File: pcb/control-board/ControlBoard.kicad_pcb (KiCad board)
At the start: 2 copper layers, 71 parts, among them J1 BOOT0, J10 Motor8, J12 Motor9, J13 Motor10, J14 JTAG-SWD, J15 HEADER_L, J16 HEADER_D, J17 HEADER_U, J18 HEADER_R, J2 Motor1, J20 PWR, J3 Motor2, J4 Motor3, J5 Motor4, J6 Motor5, J7 Motor6, J8 Motor7, J9 USB_B_Micro, SW1 RST_BTN, U1 STM32F427VGTx, U2 USBLC6-2SC6, U3 MCP1700-3302E_SOT89, U4 FT230XS, Y1 8MHz, Y2 32.768kHz

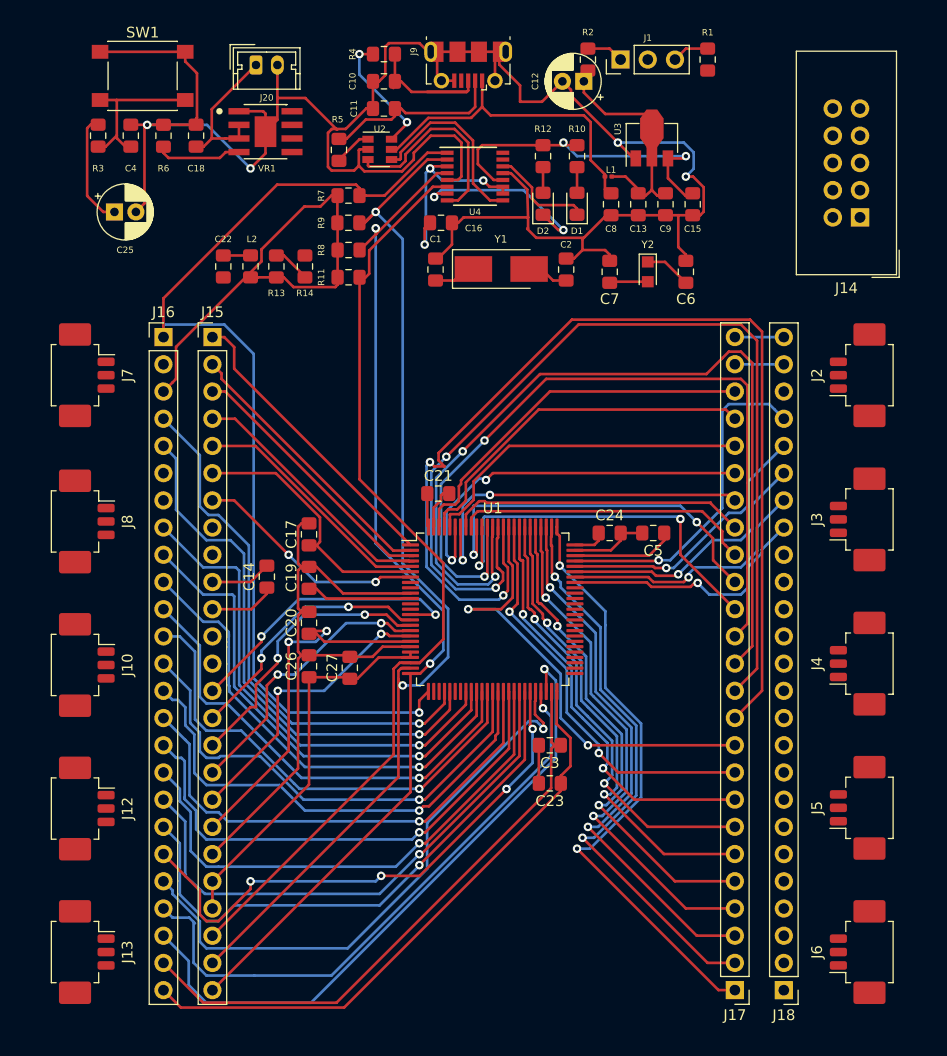
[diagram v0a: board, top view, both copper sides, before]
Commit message: Finish control board pcb
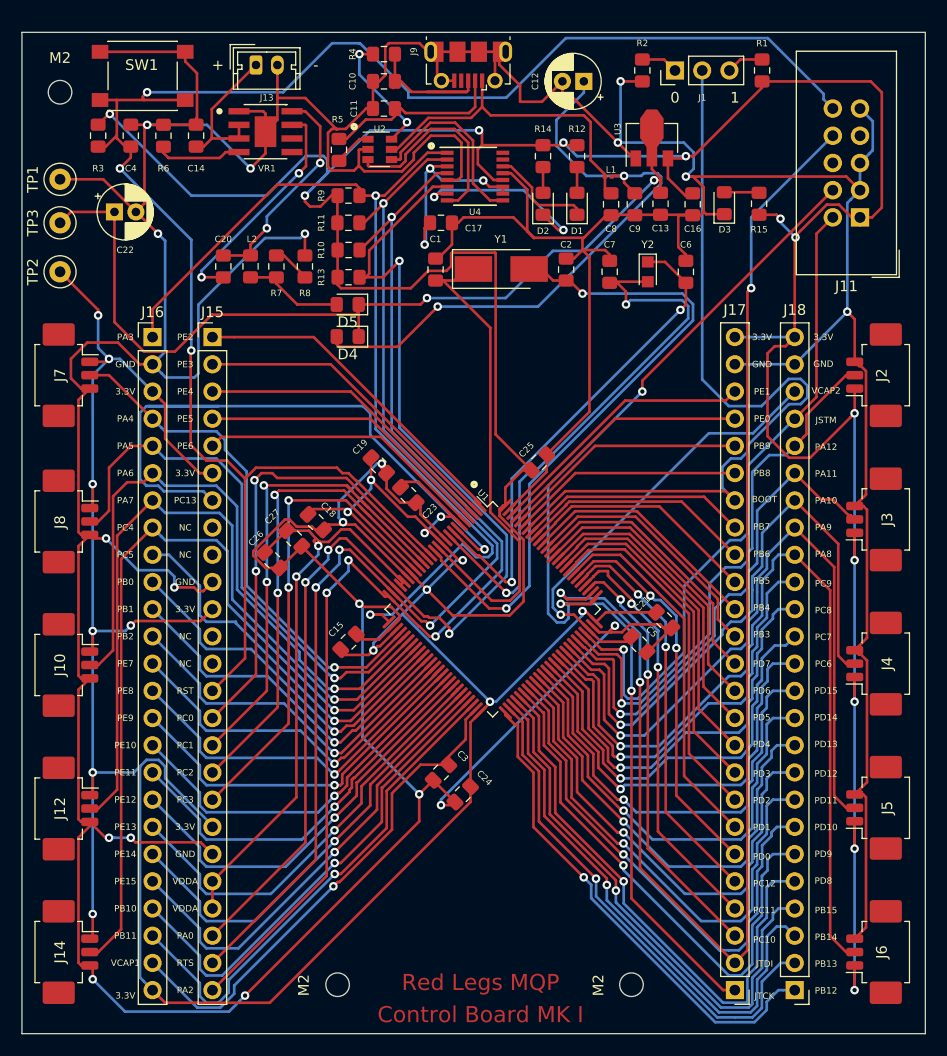
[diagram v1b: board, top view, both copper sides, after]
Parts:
- removed the C17 at (166.0, 97.7)
- removed the C23 at (188.5, 120.9)
- added C18: 100nF, Capacitor_SMD:C_0805_2012Metric_Pad1.15x1.40mm_HandSolder, F.Cu at (166.6, 96.5)
- added C24: 100nF, Capacitor_SMD:C_0805_2012Metric_Pad1.15x1.40mm_HandSolder, F.Cu at (180.3, 121.9)
- added D3: LED, LED_SMD:LED_0805_2012Metric_Pad1.15x1.40mm_HandSolder, F.Cu at (204.8, 66.8)
- added D4: SD0805, Diode_SMD:D_0805_2012Metric_Pad1.15x1.40mm_HandSolder, F.Cu at (169.6, 79.2)
- added D5: SD0805, Diode_SMD:D_0805_2012Metric_Pad1.15x1.40mm_HandSolder, F.Cu at (169.6, 76.2)
- added M2: MountingHole_2.2mm_M2, MountingHole:MountingHole_2.2mm_M2, F.Cu at (196.1, 139.7)
- added M2: MountingHole_2.2mm_M2, MountingHole:MountingHole_2.2mm_M2, F.Cu at (168.7, 139.7)
- added M2: MountingHole_2.2mm_M2, MountingHole:MountingHole_2.2mm_M2, F.Cu at (142.7, 56.4)
- added R15: 220, Resistor_SMD:R_0805_2012Metric_Pad1.15x1.40mm_HandSolder, F.Cu at (208.0, 66.8)
- added TP1: TestPoint, TestPoint:TestPoint_Loop_D2.50mm_Drill1.0mm, F.Cu at (142.7, 64.5)
- added TP2: TestPoint, TestPoint:TestPoint_Loop_D2.50mm_Drill1.0mm, F.Cu at (142.7, 73.2)
- added TP3: TestPoint, TestPoint:TestPoint_Loop_D2.50mm_Drill1.0mm, F.Cu at (142.7, 68.6)
- R12: renamed from R10; value R -> 220
- R14: renamed from R12; value R -> 220
- moved C21 33.1 mm to (199.1, 105.7), turned to 315 degrees
- moved C27 13.1 mm to (164.6, 98.0), turned to 315 degrees
- moved C19 12.4 mm to (172.5, 91.2), turned to 315 degrees
- moved C26 10.5 mm to (162.6, 100.1), turned to 315 degrees
- moved C3 10.5 mm to (178.3, 119.9), turned to 225 degrees
- moved C5 10.5 mm to (196.8, 107.9), turned to 315 degrees
- moved C15 9.75 mm to (169.7, 107.7), turned to 45 degrees
- moved C25 9.34 mm to (187.5, 90.9), turned to 45 degrees
- moved R1 5.18 mm to (208.3, 54.4)
- moved R2 5.18 mm to (197.1, 54.4)
- moved J1 5.18 mm to (200.2, 54.4)
- moved C9 2.86 mm to (196.4, 66.8)
- moved C23 2.80 mm to (175.3, 94.0), turned to 315 degrees
- moved C13 2.08 mm to (198.8, 66.8)
- moved J10 1.52 mm to (143.1, 109.9)
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- renumbered C18 to C14, C14 to C15, C15 to C16, C16 to C17, C22 to C20, C20 to C21, C25 to C22, C21 to C23, C24 to C25, J14 to J11, J20 to J13, J13 to J14, R8 to R10, R9 to R11, R11 to R13, R13 to R7, R14 to R8, R7 to R9
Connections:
- C12 pad 1: 5V -> Net-(C12-Pad1)
- C22 pad 1: 3.3V -> 5V
- C9 pad 1: 5V -> Net-(C12-Pad1)
- J10 pad 2: PD7 -> PA6
- J12 pad 2: PD8 -> PA7
- J14 pad 2: PD9 -> PC4
- J2 pad 2: PD0 -> PA12
- J3 pad 2: PD1 -> PA11
- J4 pad 2: PD2 -> PA10
- J5 pad 2: PD3 -> PA9
- J6 pad 2: PD4 -> PA8
- J7 pad 2: PD5 -> PA4
- J8 pad 2: PD6 -> PA5
- L1 pad 2: 5V -> Net-(C12-Pad1)
- L2 pad 2: 3.3V -> Net-(D5-Pad2)
- R7 pad 1: 3.3V -> Net-(D5-Pad2)
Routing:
- net GND: track 284.3 -> 669.2 mm, vias 4 -> 20
- net 3.3V: track 231.8 -> 594.6 mm, vias 4 -> 28
- net nJRST: track 42.9 -> 169.5 mm, vias 2 -> 3
- net PA8: track 0.00 -> 79.3 mm, vias 0 -> 1
- net JTDI: track 54.1 -> 127.8 mm, vias 2 -> 3
- net PD5: track 101.2 -> 28.8 mm, vias 2 -> 0
- net PA7: track 0.00 -> 69.7 mm, vias 0 -> 1
- net 5V: track 21.8 -> 85.1 mm, vias 0 -> 2
- net PD6: track 92.2 -> 29.2 mm, vias 2 -> 0
- net PA6: track 0.00 -> 60.7 mm, vias 0 -> 1
- net Net-(C12-Pad1): track 0.00 -> 59.5 mm, vias 0 -> 2
- net Net-(C2-Pad1): track 3.90 -> 61.4 mm, vias 0 -> 2
- net PD7: track 82.9 -> 25.8 mm, vias 2 -> 0
- net PD8: track 0.00 -> 52.9 mm, vias 0 -> 1
- net Net-(C7-Pad2): track 3.60 -> 54.8 mm, vias 0 -> 2
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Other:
- board outline added: 84.3 x 93.5 mm
- net class Default: clearance 0.2 -> 0.127
- rule trace_clearance: 0.2 -> 0.127
- rule trace_min: 0.2 -> 0.127
- board text added: "+"
- board text added: "-"
- board text added: "0"
- board text added: "1"
- board text added: "3.3V"
- board text added: "BOOT"
- board text added: "Control Board MK I"
- board text added: "GND"
- board text added: "JSTM"
- board text added: "JTCK"
- board text added: "JTDI"
- board text added: "NC"
- board text added: "PA0"
- board text added: "PA10"
- board text added: "PA11"
- board text added: "PA12"
- board text added: "PA2"
- board text added: "PA3"
- board text added: "PA4"
- board text added: "PA5"
- board text added: "PA6"
- board text added: "PA7"
- board text added: "PA8"
- board text added: "PA9"
- board text added: "PB0"
- board text added: "PB1"
- board text added: "PB10"
- board text added: "PB11"
- board text added: "PB12"
- board text added: "PB13"
- board text added: "PB14"
- board text added: "PB15"
- board text added: "PB2"
- board text added: "PB3"
- board text added: "PB4"
- board text added: "PB5"
- board text added: "PB6"
- board text added: "PB7"
- board text added: "PB8"
- board text added: "PB9"
- board text added: "PC0"
- board text added: "PC1"
- board text added: "PC10"
- board text added: "PC11"
- board text added: "PC12"
- board text added: "PC13"
- board text added: "PC2"
- board text added: "PC3"
- board text added: "PC4"
- board text added: "PC5"
- board text added: "PC6"
- board text added: "PC7"
- board text added: "PC8"
- board text added: "PC9"
- board text added: "PD0"
- board text added: "PD1"
- board text added: "PD10"
- board text added: "PD11"
- board text added: "PD12"
- board text added: "PD13"
- board text added: "PD14"
- board text added: "PD15"
- board text added: "PD2"
- board text added: "PD3"
- board text added: "PD4"
- board text added: "PD5"
- board text added: "PD6"
- board text added: "PD7"
- board text added: "PD8"
- board text added: "PD9"
- board text added: "PE0"
- board text added: "PE1"
- board text added: "PE10"
- board text added: "PE11"
- board text added: "PE12"
- board text added: "PE13"
- board text added: "PE14"
- board text added: "PE15"
- board text added: "PE2"
- board text added: "PE3"
- board text added: "PE4"
- board text added: "PE5"
- board text added: "PE6"
- board text added: "PE7"
- board text added: "PE8"
- board text added: "PE9"
- board text added: "RST"
- board text added: "RTS"
- board text added: "Red Legs MQP"
- board text added: "VCAP1"
- board text added: "VCAP2"
- board text added: "VDDA"
